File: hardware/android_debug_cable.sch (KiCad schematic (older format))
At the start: 12 parts, among them P1 USB_A, P2 CONN_01X04, P3 SJ-43514-SMT-TR, U1 TPS71718DCKR, U2 CP2103-GM

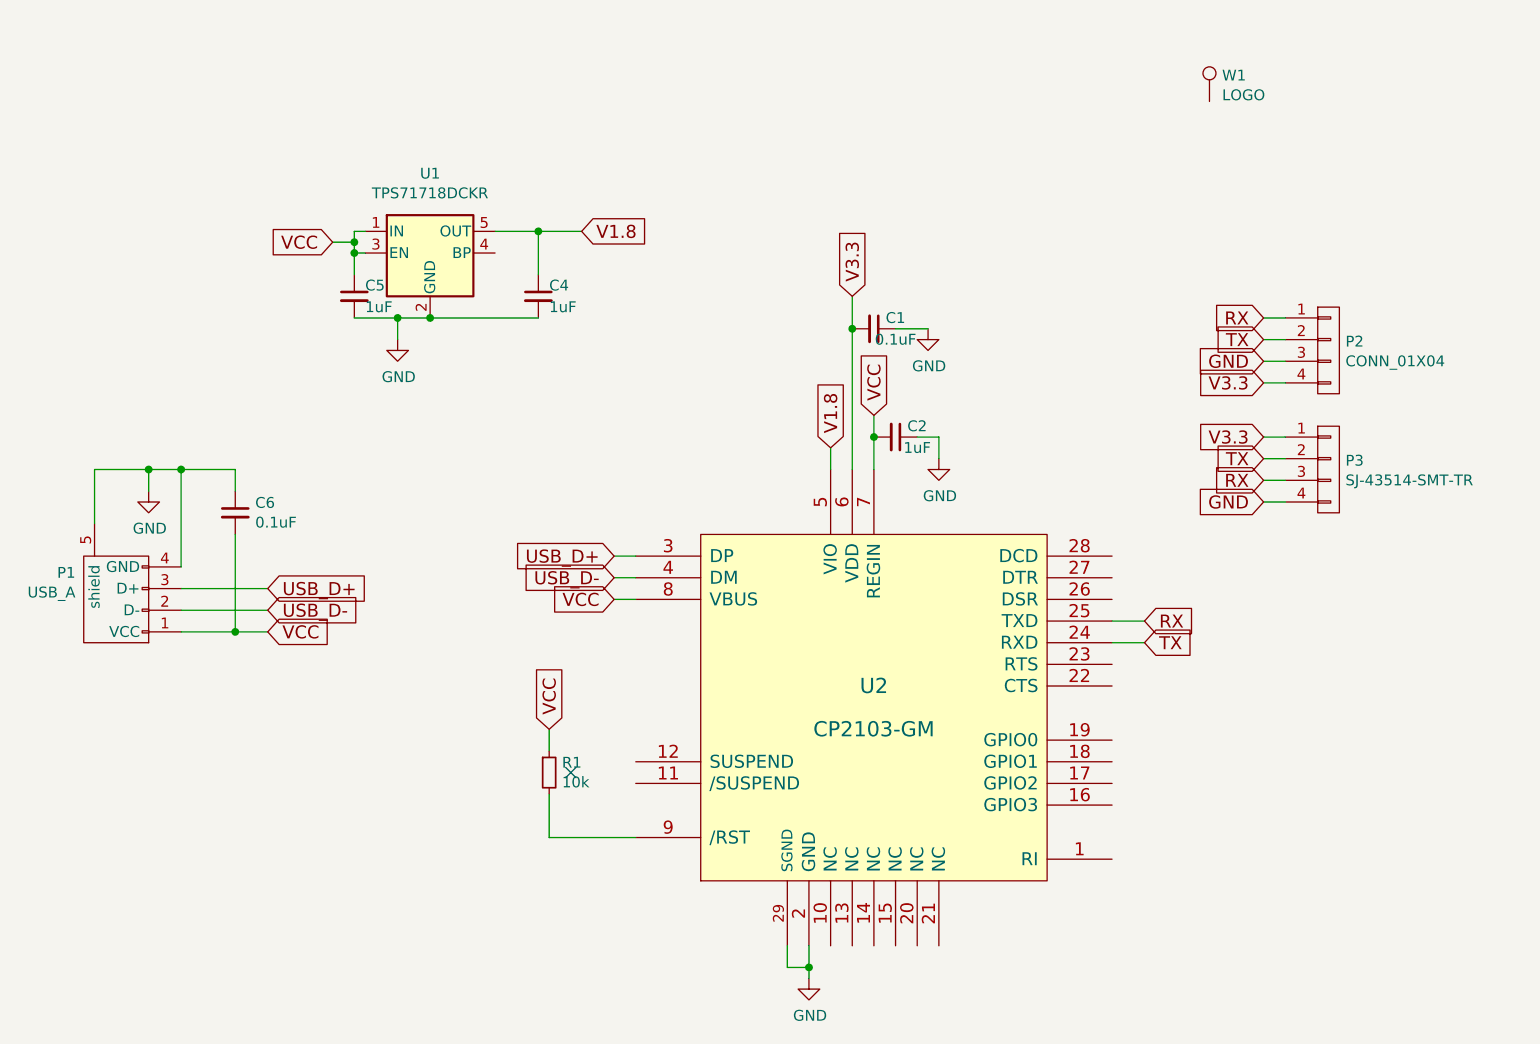
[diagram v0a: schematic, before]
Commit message: Add first version of v0.4
Signed-off-by: Robert Foss <robert.foss@collabora.com>
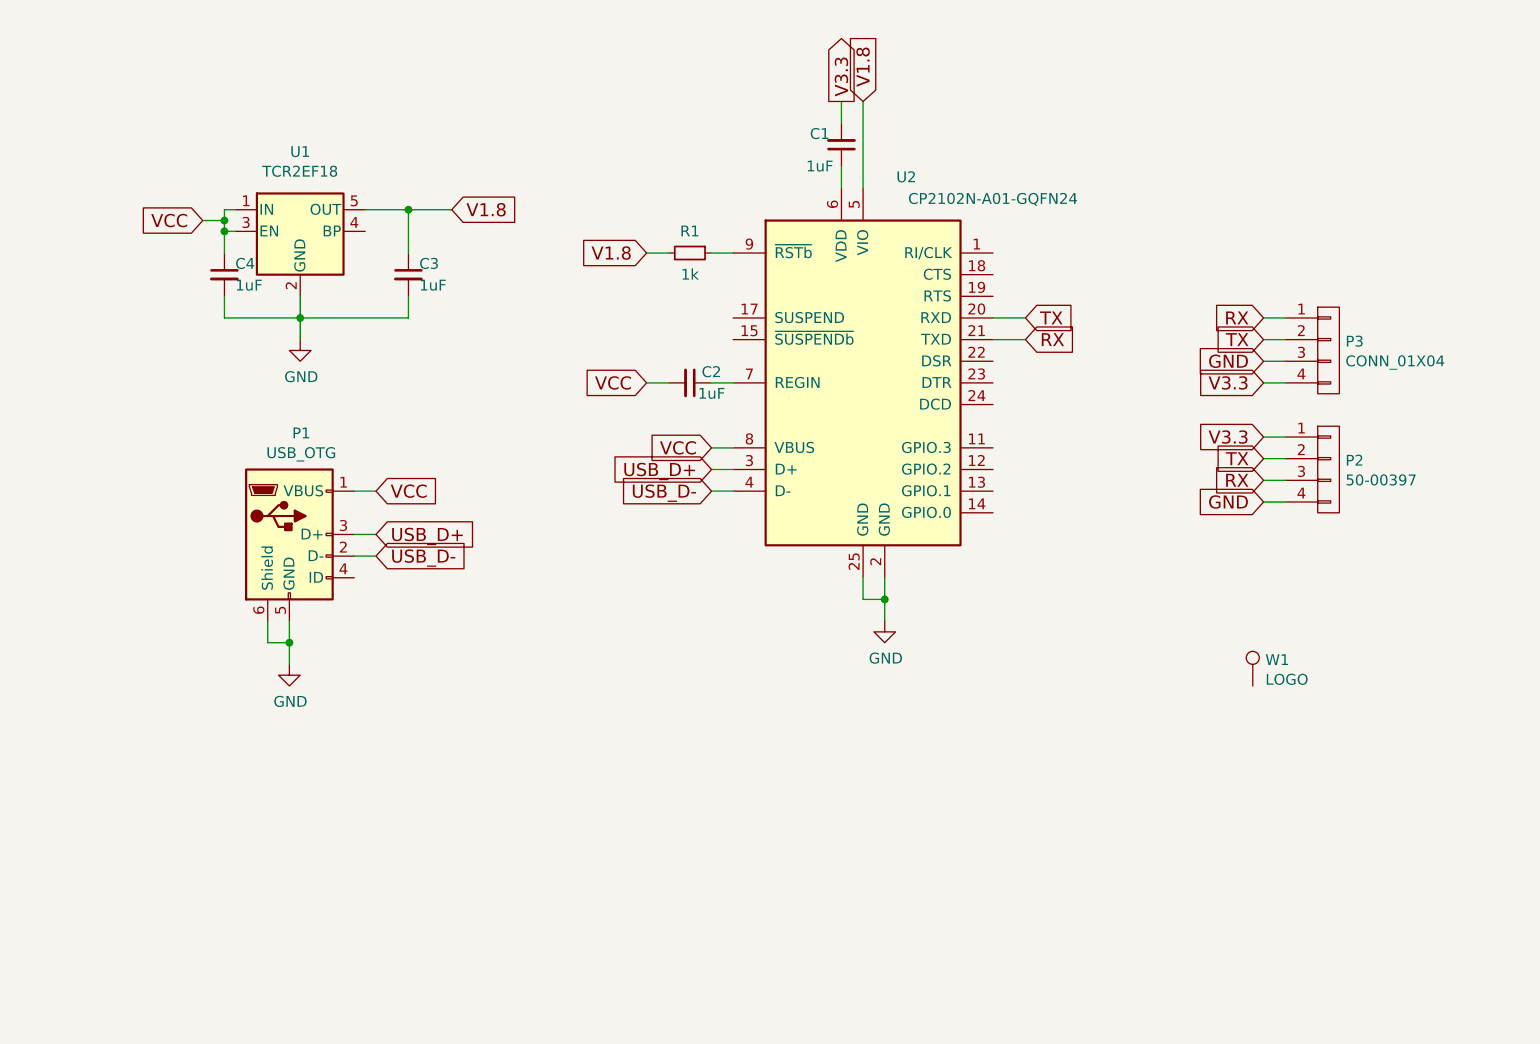
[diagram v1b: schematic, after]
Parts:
- removed C6: 0.1uF, Capacitors_SMD:C_0402, symbol C_Small
- removed P1: USB_A, connectors:usb-PCB, symbol USB_A
- removed U2: CP2103-GM, Housings_DFN_QFN:QFN-28-1EP_5x5mm_Pitch0.5mm, symbol cp2103
- added P1: USB_OTG, Connectors:USB_Micro-B, symbol USB_OTG
- added U2: CP2102N-A01-GQFN24, Housings_DFN_QFN:QFN-24-1EP_4x4mm_Pitch0.5mm, symbol CP2102N-A01-GQFN24
- C1: value 0.1uF -> 1uF
- P2: renamed from P3; value SJ-43514-SMT-TR -> 50-00397; footprint 3-5mm_4pole_jack:3.5mm_4pin_jack -> 50-00397:50-00397
- R1: value 10k -> 1k
- U1: value TPS71718DCKR -> TCR2EF18; footprint TO_SOT_Packages_SMD:SC-70-5 -> TO_SOT_Packages_SMD:SOT-23-5
- renumbered C4 to C3, C5 to C4, P2 to P3
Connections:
- net GND: now also P1.5 (GND), P1.6 (Shield), U2.2 (GND), U2.25 (GND); no longer C1.1, C2.1
- net RX: now also U2.21 (TXD)
- net TX: now also U2.20 (RXD)
- net USB_D+: now also P1.3 (D+), U2.3 (D+)
- net USB_D-: now also P1.2 (D-), U2.4 (D-)
- net V1.8: now also R1.2, U2.5 (VIO)
- net VCC: now also P1.1 (VBUS), U2.8 (VBUS); no longer R1.1
- new net: C1.1, U2.6 (VDD)
- new net: C2.1, U2.7 (REGIN)
- new net: R1.1, U2.9 (~RSTb)
- no-connect marks 1 -> 0
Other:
- moved on the sheet: C1, C2, C3, C4, U1, W1
